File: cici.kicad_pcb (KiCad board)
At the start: 2 copper layers, 88.4 x 132.8 mm, 47 parts, among them SW1 SW_PUSH, SW10 SW_PUSH, SW11 SW_PUSH, SW12 SW_PUSH, SW13 SW_PUSH, SW14 SW_PUSH, SW15 SW_PUSH, SW16 SW_PUSH, SW17 SW_PUSH, SW18 SW_PUSH, SW2 SW_PUSH, SW3 SW_PUSH, SW4 SW_PUSH, SW5 SW_PUSH, SW6 SW_PUSH, SW7 SW_PUSH, SW8 SW_PUSH, SW9 SW_PUSH, U1 ProMicro

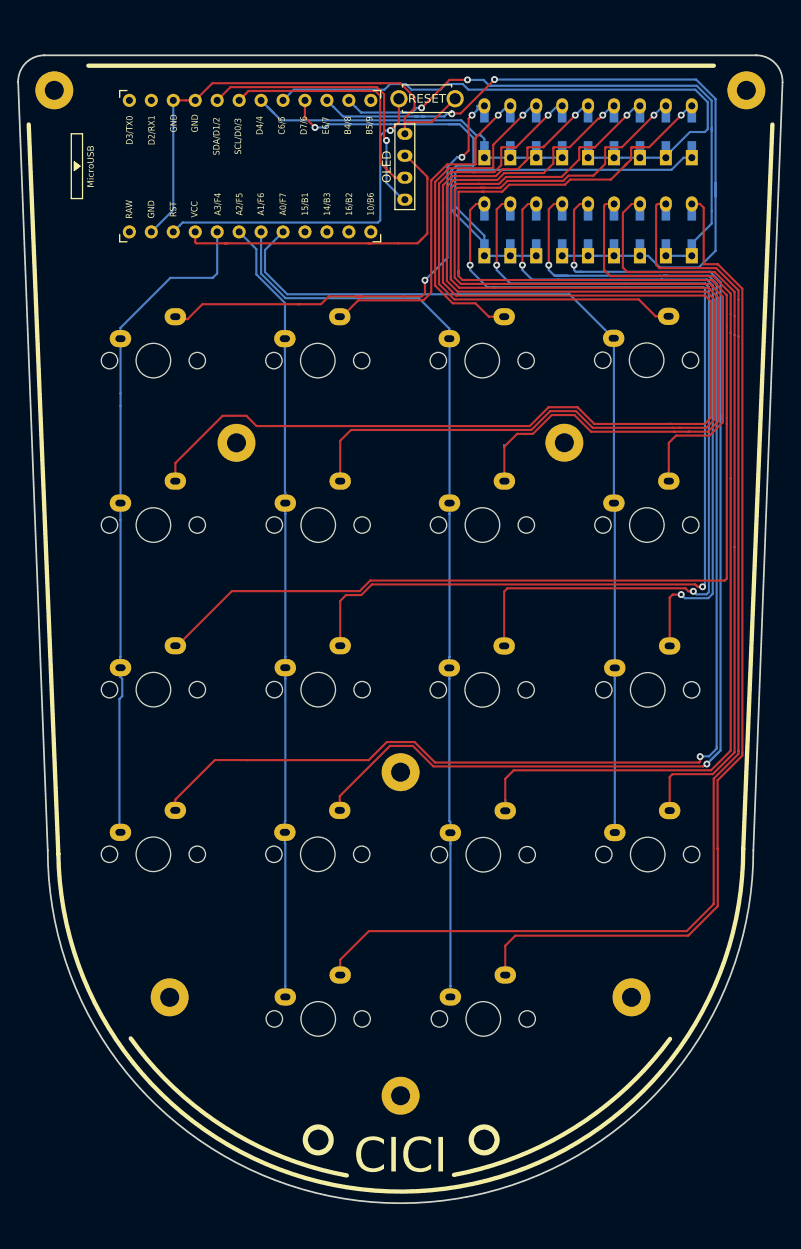
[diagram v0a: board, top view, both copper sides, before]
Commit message: creazione gerber e conclusione primo tentativo
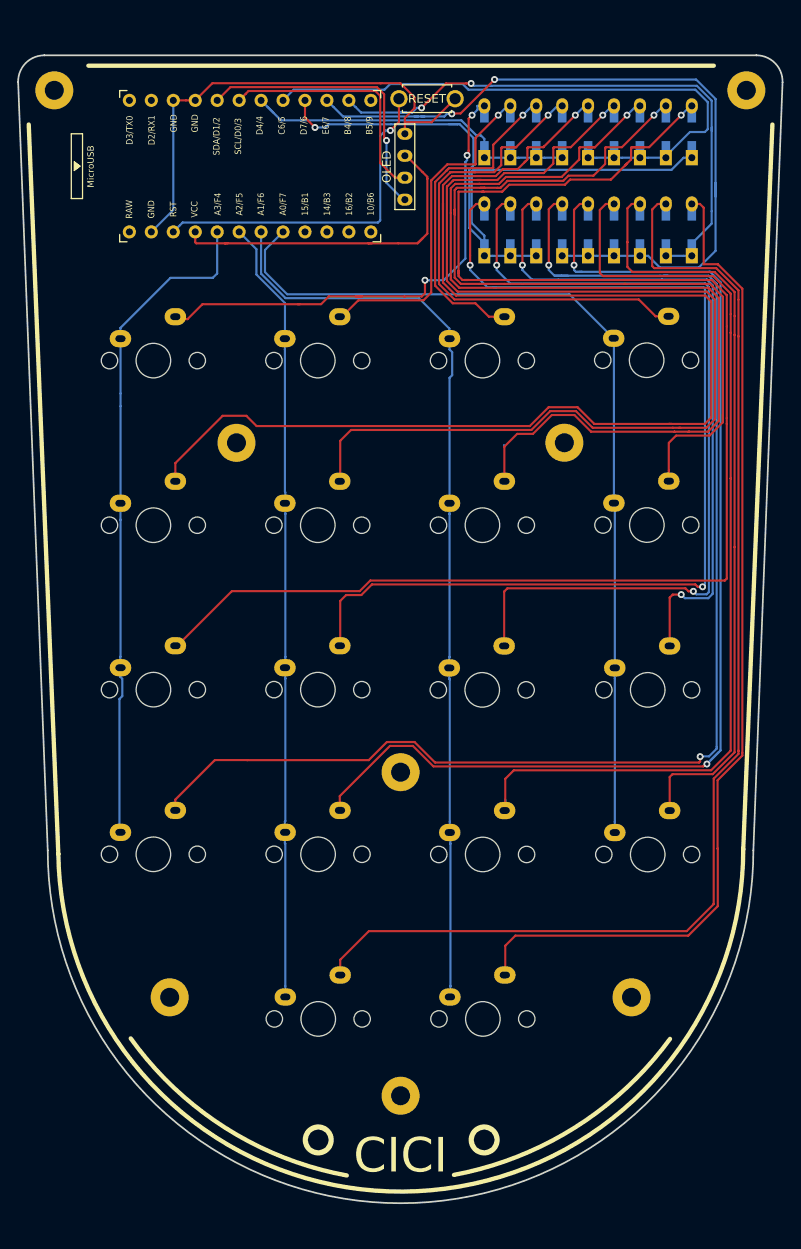
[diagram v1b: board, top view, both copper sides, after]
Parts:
- moved SW15 0.08 mm to (103.6, 118.5)
- moved SW6 0.05 mm to (84.5, 80.4)
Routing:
- net row2: track 90.2 -> 84.7 mm
- net Net-(D1-Pad2): track 57.6 -> 58.8 mm
- net Net-(D15-Pad2): track 111.0 -> 111.9 mm
- net Net-(D16-Pad2): track 89.9 -> 89.1 mm
- net Net-(D17-Pad2): track 139.9 -> 140.6 mm
- net row1: track 74.7 -> 74.1 mm

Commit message: prima versione conclusa. inizio seconda
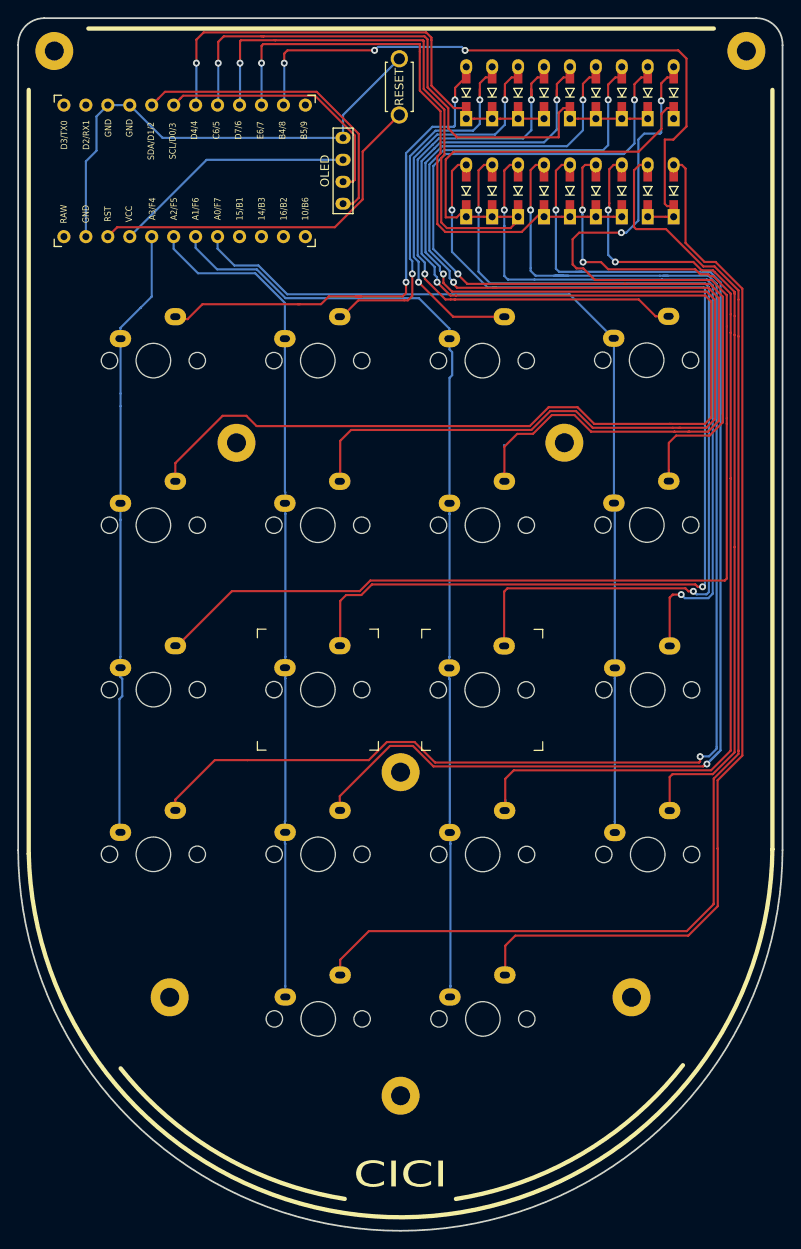
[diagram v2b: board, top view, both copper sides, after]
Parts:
- removed Ref** (x7), e: Val**, MountingHole:MountingHole_2.2mm_M2_Pad
- added REF**: MountingHole_2.2mm_M2_Pad, MountingHole:MountingHole_2.2mm_M2_Pad, F.Cu at (54.1, 25.5)
- added REF**: MountingHole_2.2mm_M2_Pad, MountingHole:MountingHole_2.2mm_M2_Pad, F.Cu at (94.1, 109.0)
- added REF**: MountingHole_2.2mm_M2_Pad, MountingHole:MountingHole_2.2mm_M2_Pad, F.Cu at (75.1, 70.8)
- added REF**: MountingHole_2.2mm_M2_Pad, MountingHole:MountingHole_2.2mm_M2_Pad, F.Cu at (113.1, 70.8)
- added REF**: MountingHole_2.2mm_M2_Pad, MountingHole:MountingHole_2.2mm_M2_Pad, F.Cu at (94.1, 146.4)
- added REF**: MountingHole_2.2mm_M2_Pad, MountingHole:MountingHole_2.2mm_M2_Pad, F.Cu at (67.4, 135.0)
- added REF**: MountingHole_2.2mm_M2_Pad, MountingHole:MountingHole_2.2mm_M2_Pad, F.Cu at (134.1, 25.5)
- added REF**: MountingHole_2.2mm_M2_Pad, MountingHole:MountingHole_2.2mm_M2_Pad, F.Cu at (120.8, 135.0)
- D1, D10, D11, D12, D13, D14, D15, D16, D17, D18, D2, D3, D4, D5, D6, D7, D8, D9: moved to F.Cu
- moved U1 7.59 mm to (69.7, 39.4)
- moved OLED1 7.17 mm to (87.5, 43.2)
- moved D1 4.98 mm to (101.7, 30.3)
- moved D10 4.98 mm to (101.7, 41.7)
- moved D11 4.98 mm to (104.7, 41.7)
- moved D12 4.98 mm to (107.7, 41.7)
- moved D13 4.98 mm to (110.7, 41.7)
- moved D14 4.98 mm to (113.7, 41.7)
- moved D15 4.98 mm to (116.7, 41.7)
- moved D16 4.98 mm to (119.7, 41.7)
- moved D17 4.98 mm to (122.7, 41.7)
- moved D18 4.98 mm to (125.7, 41.7)
- moved D2 4.98 mm to (104.7, 30.3)
- moved D3 4.98 mm to (107.7, 30.3)
- moved D4 4.98 mm to (110.7, 30.3)
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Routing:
- net row2: track 84.7 -> 112.8 mm
- net Net-(D9-Pad2): track 177.5 -> 153.2 mm, vias 1 -> 2
- net row3: track 92.3 -> 75.5 mm, vias 2 -> 1
- net Net-(D1-Pad2): track 58.8 -> 75.4 mm, vias 3 -> 2
- net row0: track 43.6 -> 60.2 mm, vias 0 -> 1
- net VCC: track 40.1 -> 28.4 mm
- net row4: track 69.1 -> 78.5 mm, vias 2 -> 3
- net Net-(D4-Pad2): track 61.6 -> 70.9 mm, vias 1 -> 2
- net Net-(D3-Pad2): track 40.3 -> 49.3 mm, vias 1 -> 2
- net Net-(D5-Pad2): track 150.4 -> 159.2 mm, vias 1 -> 2
- net Net-(D7-Pad2): track 117.9 -> 126.4 mm, vias 1 -> 2
- net Net-(D6-Pad2): track 133.7 -> 141.4 mm, vias 1 -> 2
- net Net-(D14-Pad2): track 134.1 -> 141.3 mm
- net Net-(D8-Pad2): track 101.3 -> 108.5 mm, vias 1 -> 2
- net Net-(D12-Pad2): track 79.9 -> 86.9 mm
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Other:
- board size 88.4 x 132.8 mm -> 88.4 x 140.3 mm
